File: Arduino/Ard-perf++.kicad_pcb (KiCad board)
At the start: 2 copper layers, 68.6 x 53.3 mm, 457 parts, among them P1 Power, P2 Analog, P3 Digital, P4 Digital, P5 CONN_01X01, P6 CONN_01X01, P7 CONN_01X01, P8 CONN_01X01

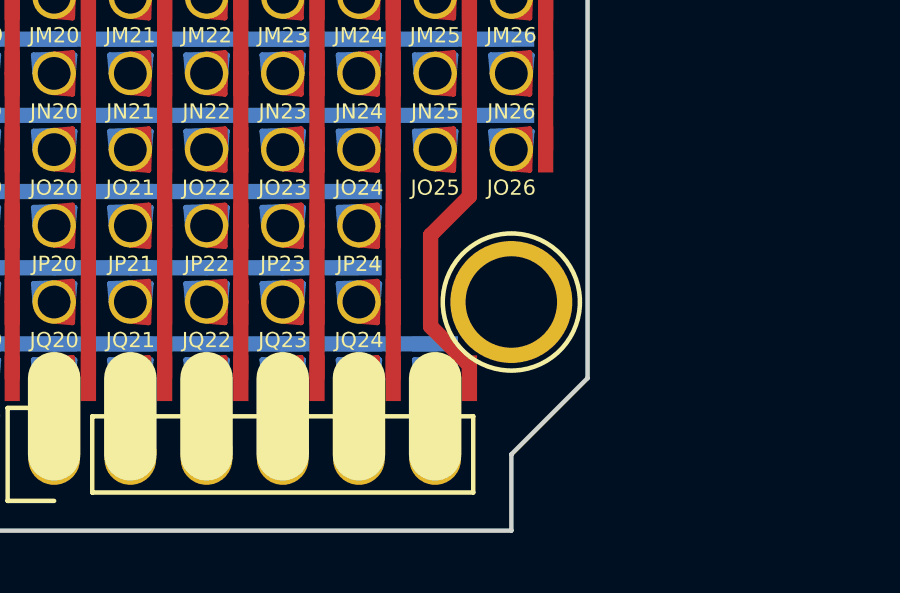
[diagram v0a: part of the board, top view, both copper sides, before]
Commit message: edit tight corner
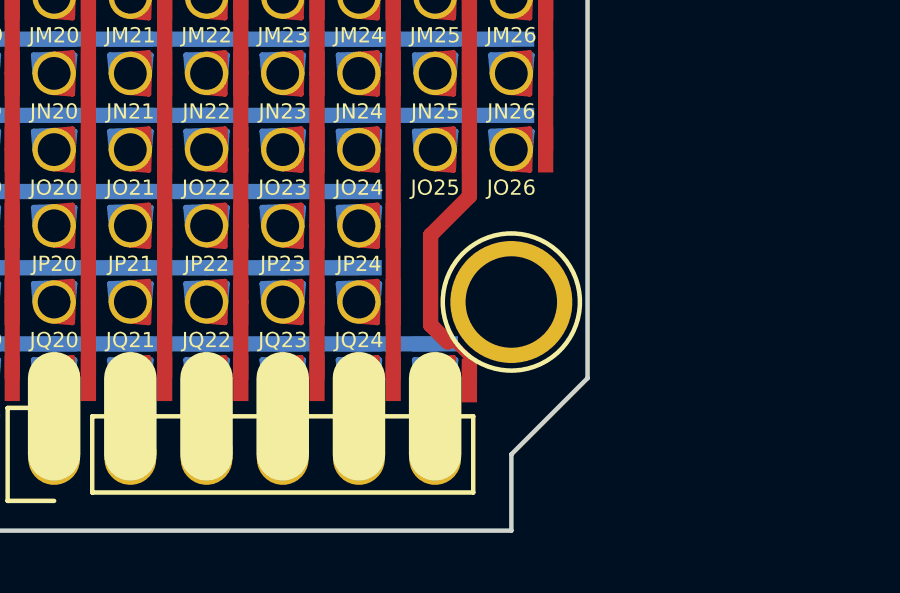
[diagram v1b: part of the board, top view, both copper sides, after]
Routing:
- net /15x25perf/J25: track 45.3 -> 46.2 mm
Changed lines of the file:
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@@
     (thickness 1.6)
     (drawings 155)
-    (tracks 931)
+    (tracks 934)
     (zones 0)
     (modules 457)
@@
     (mod_text_size 1 1)
     (mod_text_width 0.15)
-    (pad_size 4.064 4.064)
-    (pad_drill 3.048)
+    (pad_size 0.508 1.4605)
+    (pad_drill 0)
     (pad_to_mask_clearance 0)
     (aux_axis_origin 110.998 126.365)
@@
     (fp_line (start -0.6096 -0.6858) (end 0 -0.635) (layer F.Cu) (width 0.1778))
     (fp_line (start -0.635 0) (end -0.6096 -0.6858) (layer F.Cu) (width 0.1778))
-    (pad 2 smd rect (at -1.143 0 180) (size 0.508 1.524) (layers F.Cu F.Mask)
+    (pad 2 smd rect (at -1.143 -0.0762 180) (size 0.508 1.4605) (layers F.Cu F.Mask)
       (net 51 /15x25perf/J25))
     (pad 1 thru_hole circle (at 0 0 180) (size 1.4478 1.4478) (drill 1.0922) (layers *.Cu *.Mask)
@@
   (segment (start 173.101 118.745) (end 173.101 121.285) (width 0.508) (layer F.Cu) (net 49))
   (segment (start 171.958 75.565) (end 171.958 78.105) (width 0.508) (layer F.Cu) (net 50))
+  (segment (start 175.641 113.665) (end 175.641 115.2231) (width 0.508) (layer F.Cu) (net 51))
+  (segment (start 175.641 115.2231) (end 174.3456 116.5185) (width 0.508) (layer F.Cu) (net 51))
+  (segment (start 174.3456 116.5185) (end 174.3456 119.507) (width 0.508) (layer F.Cu) (net 51))
+  (segment (start 174.3456 119.507) (end 174.92218 120.08358) (width 0.508) (layer F.Cu) (net 51))
+  (segment (start 174.3456 119.5578) (end 174.5615 119.5578) (width 0.254) (layer F.Cu) (net 51))
+  (segment (start 174.5615 119.5578) (end 175.641 120.6373) (width 0.254) (layer F.Cu) (net 51))
+  (segment (start 175.641 120.6373) (end 175.641 120.8532) (width 0.254) (layer F.Cu) (net 51))
   (segment (start 175.641 85.725) (end 175.641 87.2831) (width 0.508) (layer F.Cu) (net 51))
   (segment (start 175.641 87.2831) (end 174.3964 88.5277) (width 0.508) (layer F.Cu) (net 51))
@@
   (segment (start 174.3964 92.0115) (end 175.641 93.2561) (width 0.508) (layer F.Cu) (net 51))
   (segment (start 175.641 93.2561) (end 175.641 95.885) (width 0.508) (layer F.Cu) (net 51))
-  (segment (start 175.641 113.665) (end 175.641 115.2231) (width 0.508) (layer F.Cu) (net 51))
-  (segment (start 175.641 115.2231) (end 174.3456 116.5185) (width 0.508) (layer F.Cu) (net 51))
-  (segment (start 174.3456 116.5185) (end 174.3456 119.5578) (width 0.508) (layer F.Cu) (net 51))
-  (segment (start 174.3456 119.5578) (end 175.641 120.8532) (width 0.508) (layer F.Cu) (net 51))
   (segment (start 175.641 120.8532) (end 175.641 121.285) (width 0.508) (layer F.Cu) (net 51))
   (segment (start 175.641 78.105) (end 175.641 80.645) (width 0.508) (layer F.Cu) (net 51))
